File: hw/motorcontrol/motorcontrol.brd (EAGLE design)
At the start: 65 x 58 mm, 105 parts, among them J2 USB-MICROB, U1 BTN8982TA, U10 BSS138BKS, U11 DMG2305UX, U12 BSS138BKS, U2 BTN8982TA, U3 BTN8982TA, U4 CAT24C32WI-GT3, U5 ADG3304, U6 MMDT5401, U7 PTR08060W, U8 IPD90P03P4L-04, U9 ATMEGA32U4

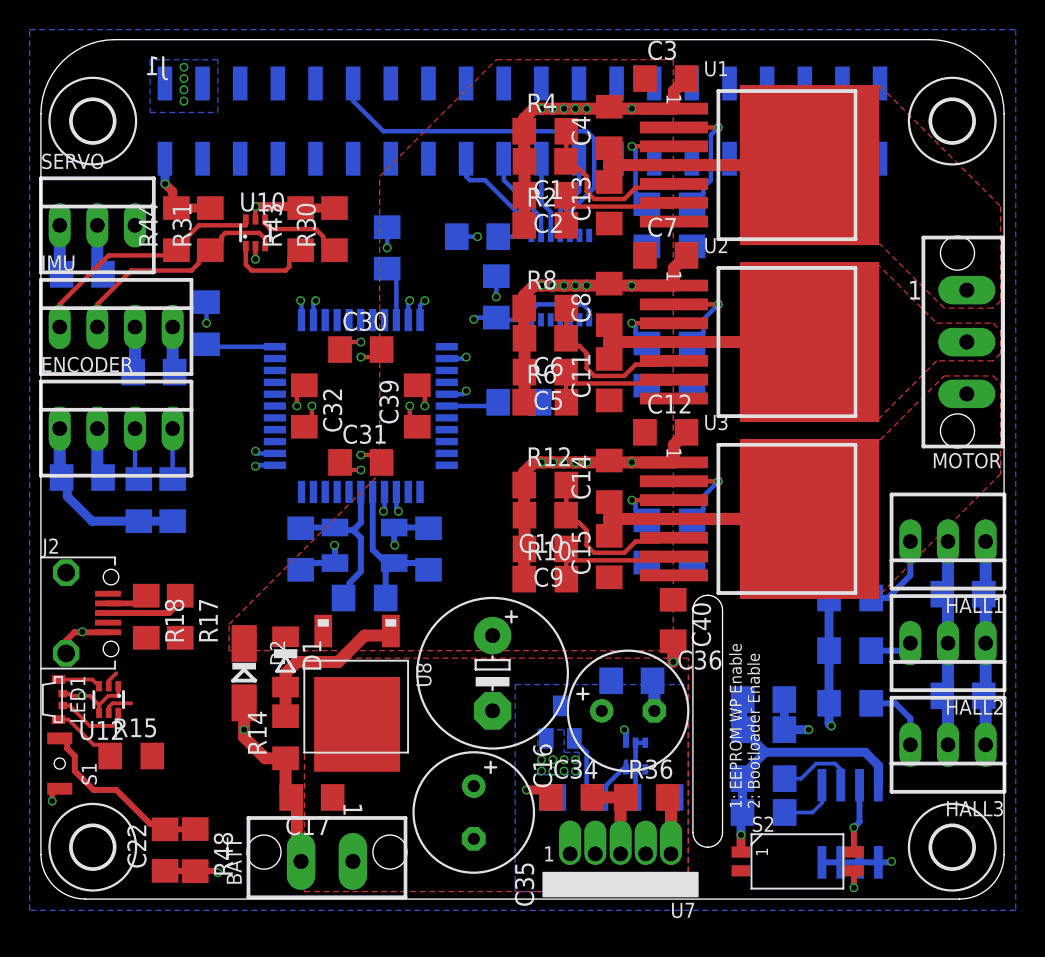
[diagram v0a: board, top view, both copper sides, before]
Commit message: backup
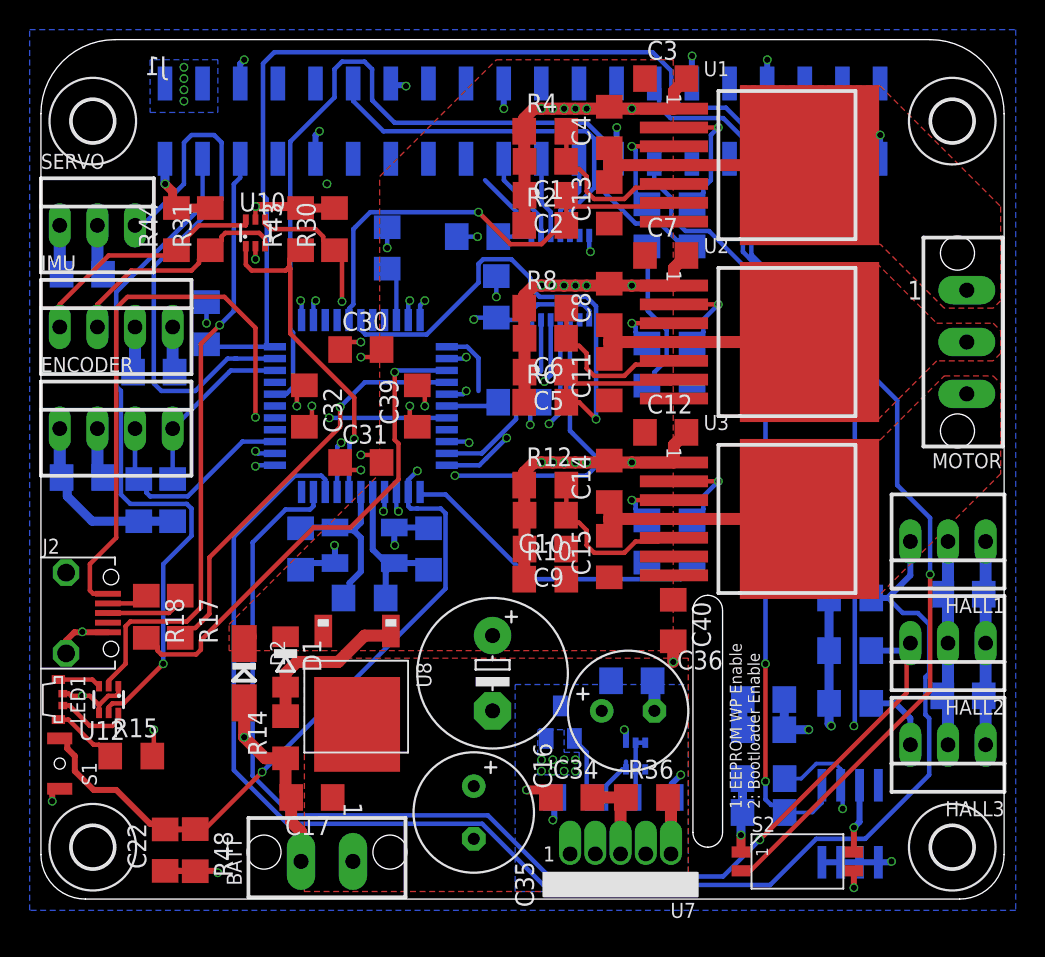
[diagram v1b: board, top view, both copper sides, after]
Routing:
- net N$8: track 4.68 -> 120.9 mm, vias 0 -> 1
- net D0: track 5.56 -> 97.2 mm
- net D1: track 2.85 -> 80.3 mm, vias 0 -> 1
- net RPIROMSCL: track 5.45 -> 64.0 mm, vias 0 -> 2
- net ATMEGARESET: track 12.6 -> 69.7 mm, vias 0 -> 3
- net D9: track 0.00 -> 57.0 mm
- net VBUS: track 0.00 -> 50.6 mm, vias 0 -> 2
- net RPIROMSDA: track 3.98 -> 52.9 mm, vias 0 -> 2
- net RPILEDG: track 2.02 -> 46.9 mm, vias 0 -> 1
- net RPILEDB: track 1.09 -> 41.5 mm, vias 0 -> 1
- net D13: track 0.00 -> 37.7 mm
- net N$23: track 0.00 -> 33.8 mm, vias 0 -> 1
- net A3: track 10.1 -> 41.4 mm, vias 0 -> 1
- net N$24: track 0.00 -> 28.2 mm, vias 0 -> 1
- net A2: track 10.1 -> 32.9 mm, vias 0 -> 1
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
